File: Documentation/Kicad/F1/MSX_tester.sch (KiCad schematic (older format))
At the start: 1 part, among them U1 BluePill

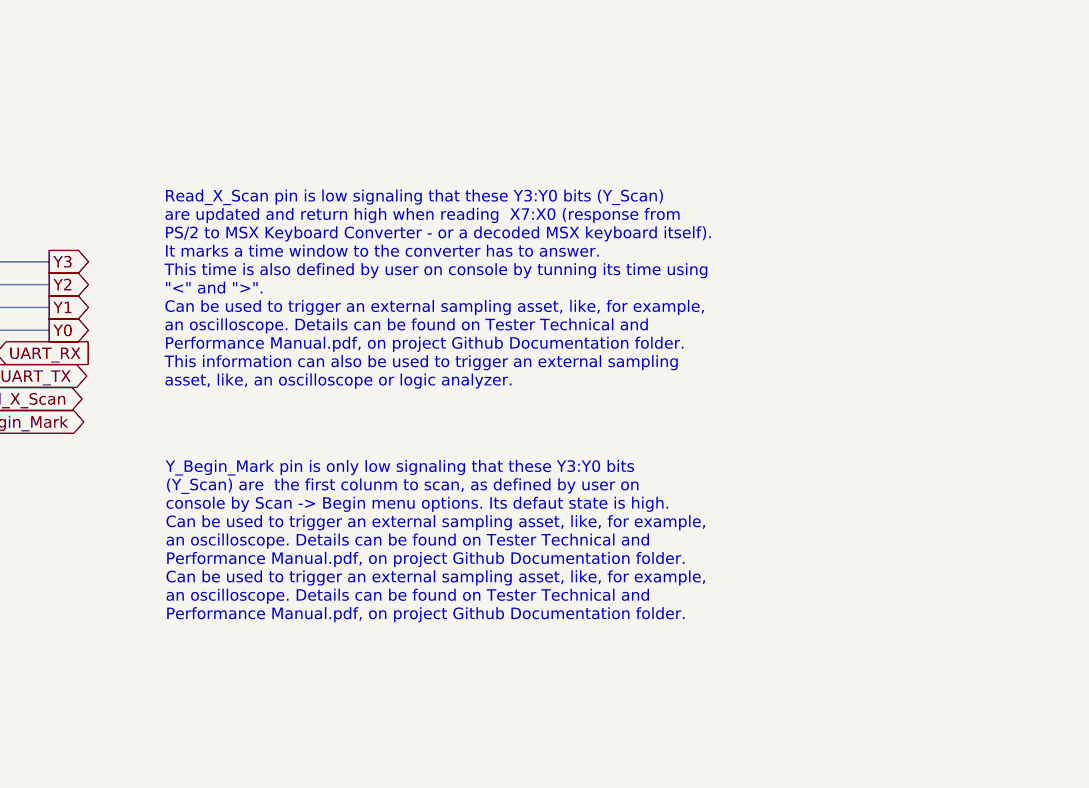
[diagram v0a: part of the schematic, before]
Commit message: Update Kicad files
Update F4 and F1 Kicad documentation
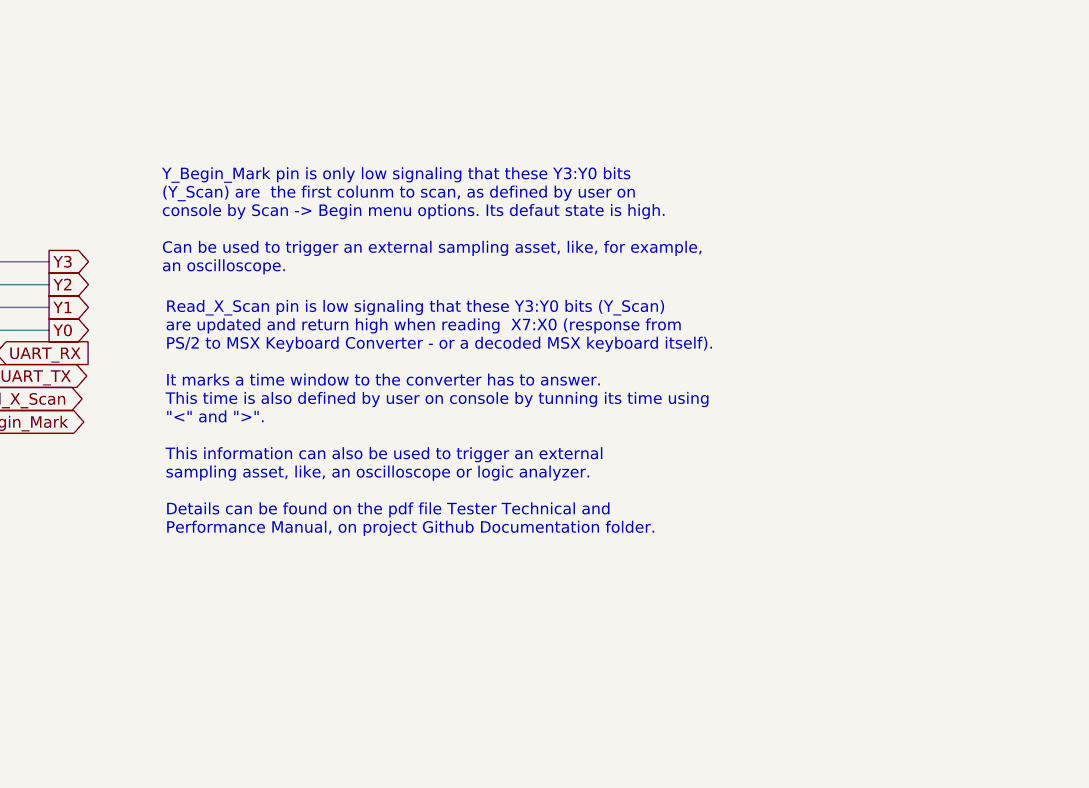
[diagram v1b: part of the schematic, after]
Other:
- note added: "Read_X_Scan pin is low signaling that these Y3:Y0 bits (Y_Scan)\nare updated and return high when reading X7:X0 (response from\nPS/2 to MSX Keyboard Converter - or a decoded MSX keyboard itself).\n\nIt marks a time window to the converter has to answer.\nThis time is also defined by user on console by tunning its time using\n"<" and ">".\n\nThis information can also be used to trigger an external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"
- note added: "Y_Begin_Mark pin is only low signaling that these Y3:Y0 bits\n(Y_Scan) are the first colunm to scan, as defined by user on\nconsole by Scan -> Begin menu options. Its defaut state is high.\n\nCan be used to trigger an external sampling asset, like, for example,\nan oscilloscope."
- note removed: "Read_X_Scan pin is low signaling that these Y3:Y0 bits (Y_Scan)\nare updated and return high when reading X7:X0 (response from\nPS/2 to MSX Keyboard Converter - or a decoded MSX keyboard itself).\nIt marks a time window to the converter has to answer.\nThis time is also defined by user on console by tunning its time using\n"<" and ">".\nCan be used to trigger an external sampling asset, like, for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"
- note removed: "Y_Begin_Mark pin is only low signaling that these Y3:Y0 bits\n(Y_Scan) are the first colunm to scan, as defined by user on\nconsole by Scan -> Begin menu options. Its defaut state is high.\nCan be used to trigger an external sampling asset, like, for example,\nan oscilloscope. Details can be found on Tester Technical and\nPerformance Manual.pdf, on project Github Documentation folder.\nCan be use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"
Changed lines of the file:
@@
 Wire Wire Line
 	2880 3518 3130 3518
-Text Notes 6540 4897 0    50   ~ 0
-Y_Begin_Mark pin is only low signaling that these Y3:Y0 bits\n(Y_Scan) are  the first colunm to scan, as defined by user on\nconsole by Scan -> Begin menu options. Its defaut state is high.\nCan be used to trigger an external sampling asset, like, for example,\nan oscilloscope. Details can be found on Tester Technical and\nPerformance Manual.pdf, on project Github Documentation folder.\nCan be used to trigger an external sampling asset, like, for example,\nan oscilloscope. Details can be found on Tester Technical and\nPerformance Manual.pdf, on project Github Documentation folder.
-Text Notes 6535 3875 0    50   ~ 0
-Read_X_Scan pin is low signaling that these Y3:Y0 bits (Y_Scan)\nare updated and return high when reading  X7:X0 (response from\nPS/2 to MSX Keyboard Converter - or a decoded MSX keyboard itself).\nIt marks a time window to the converter has to answer.\nThis time is also defined by user on console by tunning its time using\n"<" and ">".\nCan be used to trigger an external sampling asset, like, for example,\nan oscilloscope. Details can be found on Tester Technical and\nPerformance Manual.pdf, on project Github Documentation folder.\nThis information can also be used to trigger an external sampling\nasset, like, an oscilloscope or logic analyzer.
+Text Notes 6540 4519 0    50   ~ 0
+Read_X_Scan pin is low signaling that these Y3:Y0 bits (Y_Scan)\nare updated and return high when reading  X7:X0 (response from\nPS/2 to MSX Keyboard Converter - or a decoded MSX keyboard itself).\n\nIt marks a time window to the converter has to answer.\nThis time is also defined by user on console by tunning its time using\n"<" and ">".\n\nThis information can also be used to trigger an external\nsampling asset, like, an oscilloscope or logic analyzer.\n\nDetails can be found on the pdf file Tester Technical and \nPerformance Manual, on project Github Documentation folder.
+Text Notes 6524 3375 0    50   ~ 0
+Y_Begin_Mark pin is only low signaling that these Y3:Y0 bits\n(Y_Scan) are  the first colunm to scan, as defined by user on\nconsole by Scan -> Begin menu options. Its defaut state is high.\n\nCan be used to trigger an external sampling asset, like, for example,\nan oscilloscope.
 Text Notes 10746 7635 0    50   ~ 0
 1.4
